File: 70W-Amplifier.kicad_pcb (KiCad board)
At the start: 2 copper layers, 35 parts, among them J1 RF_OUT, J2 RF_IN, J3 LPF_IN, J4 LPF_OUT, J5 13.8V Input, J6 PTT, K1 G5V-2, Q1 2N3906-SMD, Q2 IRF530, Q3 IRF530, T1 BN-43-202 1T:2T, T2 Ferrite 1T:3T, U1 L7805

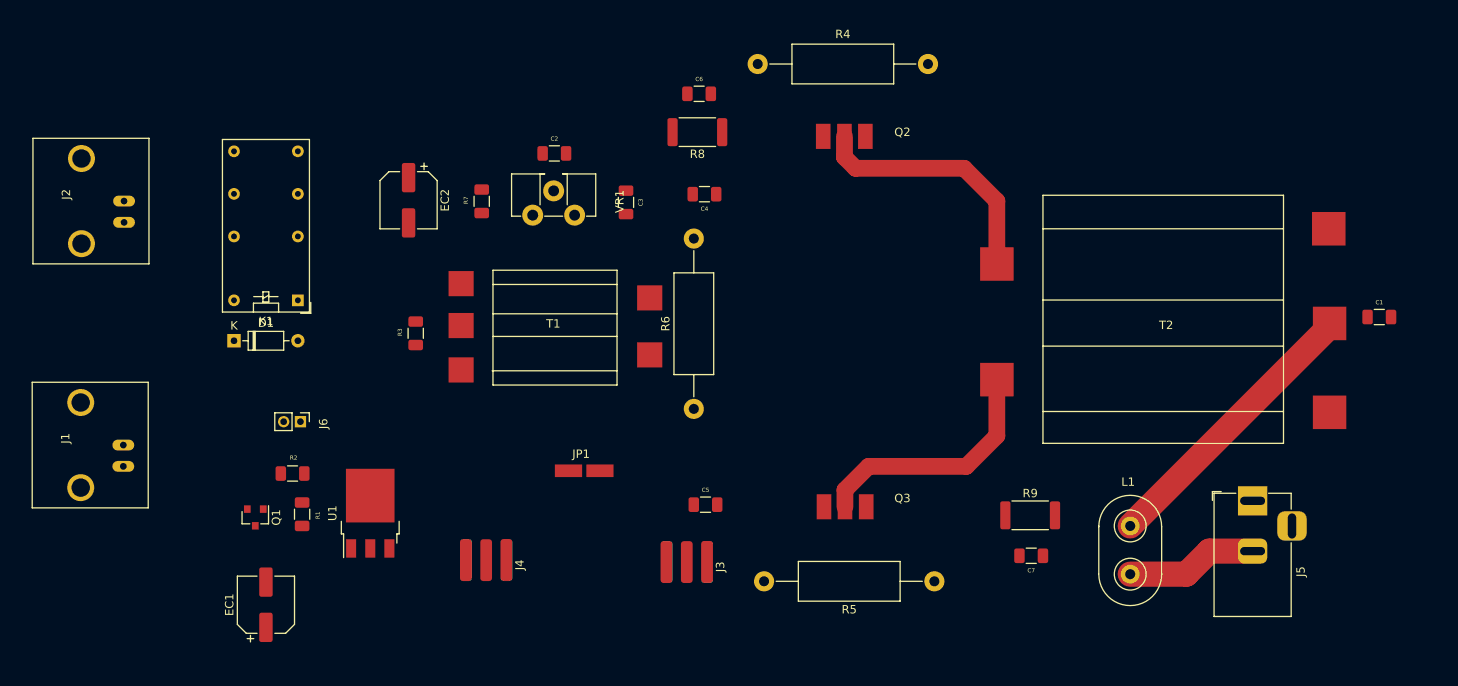
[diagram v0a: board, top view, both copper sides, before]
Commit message: Update 70W-Amplifier.kicad_pcb
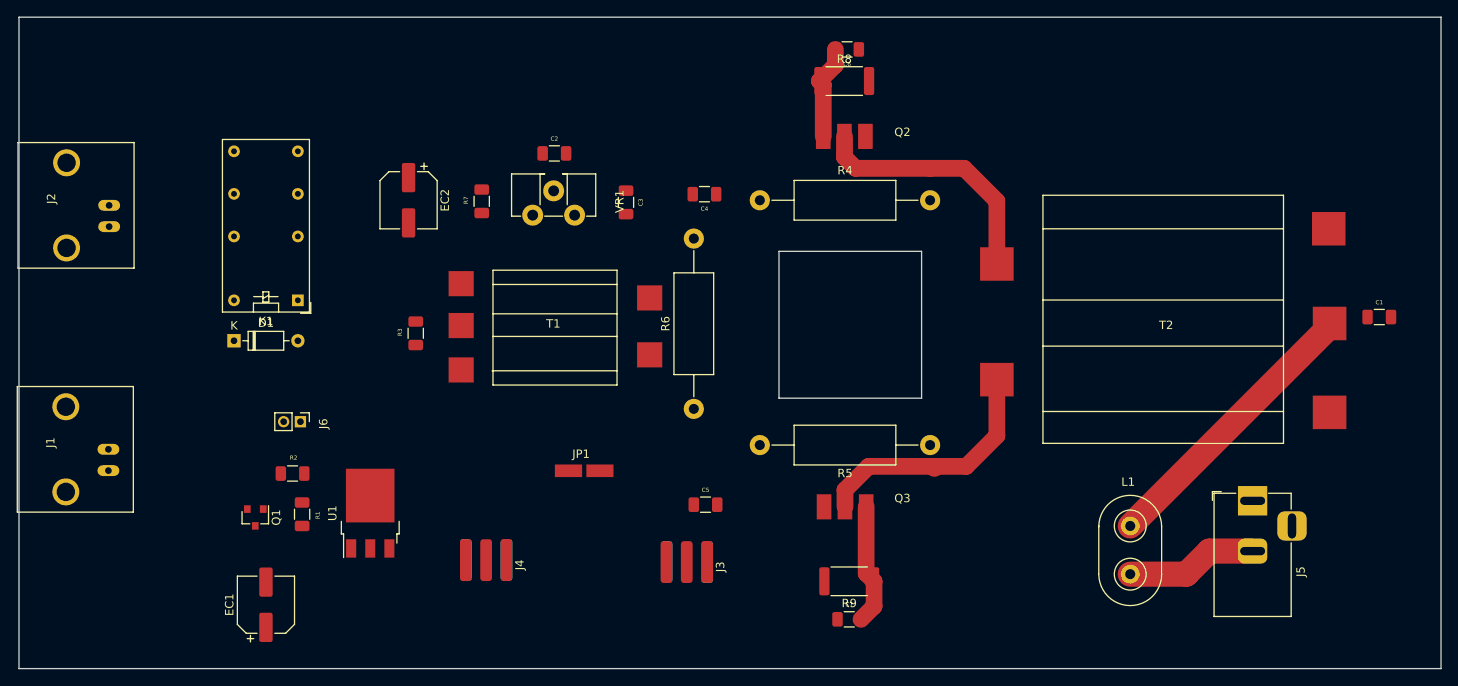
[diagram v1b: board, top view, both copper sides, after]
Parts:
- moved R9 23.0 mm to (175.8, 113.3), turned to 180 degrees
- moved C7 21.9 mm to (175.8, 115.6), turned to 0 degrees
- moved R8 18.6 mm to (175.2, 53.6), turned to 0 degrees
- moved C6 17.7 mm to (175.5, 52.1), turned to 180 degrees
- moved R5 16.3 mm to (185.4, 97.0)
- moved R4 16.3 mm to (185.4, 67.8)
- moved J1 1.85 mm to (83.5, 97.4)
- moved J2 1.85 mm to (83.6, 68.3)
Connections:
- T2 pad 1: GND -> Net-(J3-Pad1)
- T2 pad 2: Net-(J3-Pad1) -> GND
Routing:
- net Net-(C7-Pad2): track 0.00 -> 14.5 mm
- net Net-(C6-Pad2): track 0.00 -> 11.4 mm
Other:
- board outline added: 169.7 x 77.7 mm
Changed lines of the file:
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@@
   (general
     (thickness 1.6)
-    (drawings 0)
-    (tracks 15)
+    (drawings 8)
+    (tracks 26)
     (zones 0)
     (modules 35)
@@
   )
   (module Resistor_SMD:R_2512_6332Metric (layer F.Cu)
-    (at 197.358 105.41)
+    (at 175.768 113.284 180)
     (descr "Resistor SMD 2512 (6332 Metric), square (rectangular) end terminal, IPC_7351 nominal, (Body size source: IPC-SM-782 page 72, https://www.pcb-3d.com/wordpress/wp-content/uploads/ipc-sm-782a_amendment_1_and_2.pdf), generated with kicad-footprint-generator")
     (tags resistor)
@@
       (effects (font (size 1 1) (thickness 0.15)))
     )
-    (pad 2 smd roundrect (at 2.9625 0) (size 1.225 3.35) (layers F.Cu F.Paste F.Mask) (roundrect_rratio 0.204082)
-      (net 1 GND))
-    (pad 1 smd roundrect (at -2.9625 0) (size 1.225 3.35) (layers F.Cu F.Paste F.Mask) (roundrect_rratio 0.204082)
+    (pad 2 smd roundrect (at 2.9625 0 180) (size 1.225 3.35) (layers F.Cu F.Paste F.Mask) (roundrect_rratio 0.204082)
+      (net 1 GND))
+    (pad 1 smd roundrect (at -2.9625 0 180) (size 1.225 3.35) (layers F.Cu F.Paste F.Mask) (roundrect_rratio 0.204082)
       (net 23 "Net-(C7-Pad2)"))
     (model ${KISYS3DMOD}/Resistor_SMD.3dshapes/R_2512_6332Metric.wrl
@@
   )
   (module Resistor_SMD:R_2512_6332Metric (layer F.Cu)
-    (at 157.6485 59.69 180)
+    (at 175.1745 53.594)
     (descr "Resistor SMD 2512 (6332 Metric), square (rectangular) end terminal, IPC_7351 nominal, (Body size source: IPC-SM-782 page 72, https://www.pcb-3d.com/wordpress/wp-content/uploads/ipc-sm-782a_amendment_1_and_2.pdf), generated with kicad-footprint-generator")
     (tags resistor)
@@
       (effects (font (size 1 1) (thickness 0.15)))
     )
-    (pad 2 smd roundrect (at 2.9625 0 180) (size 1.225 3.35) (layers F.Cu F.Paste F.Mask) (roundrect_rratio 0.204082)
-      (net 1 GND))
-    (pad 1 smd roundrect (at -2.9625 0 180) (size 1.225 3.35) (layers F.Cu F.Paste F.Mask) (roundrect_rratio 0.204082)
+    (pad 2 smd roundrect (at 2.9625 0) (size 1.225 3.35) (layers F.Cu F.Paste F.Mask) (roundrect_rratio 0.204082)
+      (net 1 GND))
+    (pad 1 smd roundrect (at -2.9625 0) (size 1.225 3.35) (layers F.Cu F.Paste F.Mask) (roundrect_rratio 0.204082)
       (net 22 "Net-(C6-Pad2)"))
     (model ${KISYS3DMOD}/Resistor_SMD.3dshapes/R_2512_6332Metric.wrl
@@
   )
   (module "Xenir:Capacitor 1206" (layer F.Cu)
-    (at 197.482 112.486 180)
+    (at 175.768 115.57)
     (fp_text reference C7 (at 0 0.5) (layer F.SilkS)
       (effects (font (size 0.5 0.5) (thickness 0.125)))
@@
       (effects (font (size 0.8 0.8) (thickness 0.12)))
     )
-    (pad 2 smd roundrect (at 1.4 2.25 180) (size 1.25 1.75) (layers F.Cu F.Paste F.Mask) (roundrect_rratio 0.2)
+    (pad 2 smd roundrect (at 1.4 2.25) (size 1.25 1.75) (layers F.Cu F.Paste F.Mask) (roundrect_rratio 0.2)
       (net 23 "Net-(C7-Pad2)"))
-    (pad 1 smd roundrect (at -1.4 2.25 180) (size 1.25 1.75) (layers F.Cu F.Paste F.Mask) (roundrect_rratio 0.2)
+    (pad 1 smd roundrect (at -1.4 2.25) (size 1.25 1.75) (layers F.Cu F.Paste F.Mask) (roundrect_rratio 0.2)
       (net 1 GND))
   )
   (module "Xenir:Capacitor 1206" (layer F.Cu)
-    (at 157.858 52.868)
+    (at 175.514 52.07 180)
     (fp_text reference C6 (at 0 0.5) (layer F.SilkS)
       (effects (font (size 0.5 0.5) (thickness 0.125)))
@@
       (effects (font (size 0.8 0.8) (thickness 0.12)))
     )
-    (pad 2 smd roundrect (at 1.4 2.25) (size 1.25 1.75) (layers F.Cu F.Paste F.Mask) (roundrect_rratio 0.2)
+    (pad 2 smd roundrect (at 1.4 2.25 180) (size 1.25 1.75) (layers F.Cu F.Paste F.Mask) (roundrect_rratio 0.2)
       (net 22 "Net-(C6-Pad2)"))
-    (pad 1 smd roundrect (at -1.4 2.25) (size 1.25 1.75) (layers F.Cu F.Paste F.Mask) (roundrect_rratio 0.2)
+    (pad 1 smd roundrect (at -1.4 2.25 180) (size 1.25 1.75) (layers F.Cu F.Paste F.Mask) (roundrect_rratio 0.2)
       (net 1 GND))
   )
@@
   )
   (module Resistor_THT:R_Axial_DIN0414_L11.9mm_D4.5mm_P20.32mm_Horizontal (layer F.Cu)
-    (at 185.928 113.284 180)
+    (at 185.42 97.028 180)
     (descr "Resistor, Axial_DIN0414 series, Axial, Horizontal, pin pitch=20.32mm, 2W, length*diameter=11.9*4.5mm^2, http://www.vishay.com/docs/20128/wkxwrx.pdf")
     (tags "Resistor Axial_DIN0414 series Axial Horizontal pin pitch 20.32mm 2W length 11.9mm diameter 4.5mm")
@@
   )
   (module Resistor_THT:R_Axial_DIN0414_L11.9mm_D4.5mm_P20.32mm_Horizontal (layer F.Cu)
-    (at 185.166 51.562 180)
+    (at 185.42 67.818 180)
     (descr "Resistor, Axial_DIN0414 series, Axial, Horizontal, pin pitch=20.32mm, 2W, length*diameter=11.9*4.5mm^2, http://www.vishay.com/docs/20128/wkxwrx.pdf")
     (tags "Resistor Axial_DIN0414 series Axial Horizontal pin pitch 20.32mm 2W length 11.9mm diameter 4.5mm")
@@
       (net 21 /Q3Drain))
     (pad 2 smd rect (at -18.1 28.6 180) (size 4 4) (layers F.Cu F.Paste F.Mask)
-      (net 12 "Net-(J3-Pad1)"))
+      (net 1 GND))
     (pad 4 smd rect (at -18.2 17.3 180) (size 4 4) (layers F.Cu F.Paste F.Mask)
       (net 2 "Net-(C1-Pad1)"))
     (pad 1 smd rect (at -18.2 6.7 180) (size 4 4) (layers F.Cu F.Paste F.Mask)
-      (net 1 GND))
+      (net 12 "Net-(J3-Pad1)"))
   )
   (module Xenir:PCB-SMA-EDGE (layer F.Cu)
@@
   )
   (module Xenir:BNC (layer F.Cu)
-    (at 85.344 67.818 90)
+    (at 83.566 68.326 90)
     (fp_text reference J2 (at 0.7 -3 90) (layer F.SilkS)
       (effects (font (size 1 1) (thickness 0.15)))
@@
   )
   (module Xenir:BNC (layer F.Cu)
-    (at 85.254 96.928 90)
+    (at 83.476 97.436 90)
     (fp_text reference J1 (at 0.7 -3 90) (layer F.SilkS)
       (effects (font (size 1 1) (thickness 0.15)))
@@
       (net 2 "Net-(C1-Pad1)"))
   )
+  (gr_line (start 184.404 73.914) (end 184.404 91.44) (layer Edge.Cuts) (width 0.1))
+  (gr_line (start 167.386 73.914) (end 184.404 73.914) (layer Edge.Cuts) (width 0.1))
+  (gr_line (start 167.386 91.44) (end 167.386 73.914) (layer Edge.Cuts) (width 0.1))
+  (gr_line (start 184.404 91.44) (end 167.386 91.44) (layer Edge.Cuts) (width 0.1))
+  (gr_line (start 246.38 45.974) (end 246.38 123.698) (layer Edge.Cuts) (width 0.1))
+  (gr_line (start 76.708 45.974) (end 246.38 45.974) (layer Edge.Cuts) (width 0.1))
+  (gr_line (start 76.708 123.698) (end 76.708 45.974) (layer Edge.Cuts) (width 0.1))
+  (gr_line (start 246.38 123.698) (end 76.708 123.698) (layer Edge.Cuts) (width 0.1))
   (segment (start 233.084 82.892) (end 209.296 106.68) (width 3) (layer F.Cu) (net 2))
   (segment (start 233.084 82.522) (end 233.084 82.892) (width 3) (layer F.Cu) (net 2))
@@
   (segment (start 175.19904 60.198) (end 175.19904 62.67704) (width 2) (layer F.Cu) (net 20))
   (segment (start 175.19904 62.67704) (end 176.53 64.008) (width 2) (layer F.Cu) (net 20))
-  (segment (start 176.53 64.008) (end 189.484 64.008) (width 2) (layer F.Cu) (net 20))
   (segment (start 193.384 67.908) (end 193.384 75.422) (width 2) (layer F.Cu) (net 20))
   (segment (start 189.484 64.008) (end 193.384 67.908) (width 2) (layer F.Cu) (net 20))
+  (segment (start 185.42 64.008) (end 189.484 64.008) (width 2) (layer F.Cu) (net 20))
+  (segment (start 176.53 64.008) (end 185.42 64.008) (width 2) (layer F.Cu) (net 20))
   (segment (start 193.384 89.222) (end 193.384 95.922) (width 2) (layer F.Cu) (net 21))
   (segment (start 193.384 95.922) (end 189.738 99.568) (width 2) (layer F.Cu) (net 21))
   (segment (start 175.26 102.388838) (end 175.26 104.394) (width 2) (layer F.Cu) (net 21))
   (segment (start 178.080838 99.568) (end 175.26 102.388838) (width 2) (layer F.Cu) (net 21))
-  (segment (start 189.738 99.568) (end 178.080838 99.568) (width 2) (layer F.Cu) (net 21))
+  (segment (start 185.928 99.822) (end 185.674 99.568) (width 2) (layer F.Cu) (net 21))
+  (segment (start 185.674 99.568) (end 178.080838 99.568) (width 2) (layer F.Cu) (net 21))
+  (segment (start 189.738 99.568) (end 185.674 99.568) (width 2) (layer F.Cu) (net 21))
+  (segment (start 172.6692 54.0512) (end 172.212 53.594) (width 2) (layer F.Cu) (net 22))
+  (segment (start 172.6692 60.198) (end 172.6692 54.0512) (width 2) (layer F.Cu) (net 22))
+  (segment (start 174.114 51.692) (end 172.212 53.594) (width 2) (layer F.Cu) (net 22))
+  (segment (start 174.114 49.82) (end 174.114 51.692) (width 2) (layer F.Cu) (net 22))
+  (segment (start 177.78984 112.34334) (end 178.7305 113.284) (width 2) (layer F.Cu) (net 23))
+  (segment (start 177.78984 104.394) (end 177.78984 112.34334) (width 2) (layer F.Cu) (net 23))
+  (segment (start 178.7305 116.2575) (end 177.168 117.82) (width 2) (layer F.Cu) (net 23))
+  (segment (start 178.7305 113.284) (end 178.7305 116.2575) (width 2) (layer F.Cu) (net 23))
 )
